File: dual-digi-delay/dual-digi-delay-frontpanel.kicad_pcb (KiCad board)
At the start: 2 copper layers, 50.5 x 175 mm, 1 part

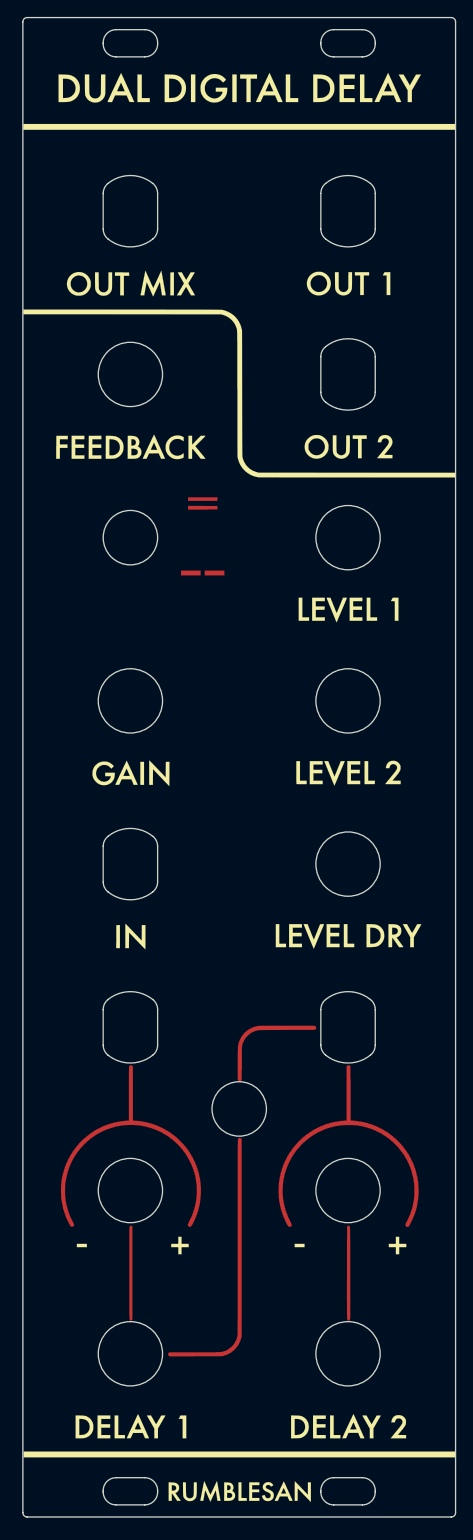
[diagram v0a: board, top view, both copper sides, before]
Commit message: Finalising rev 01 of dual digi delay
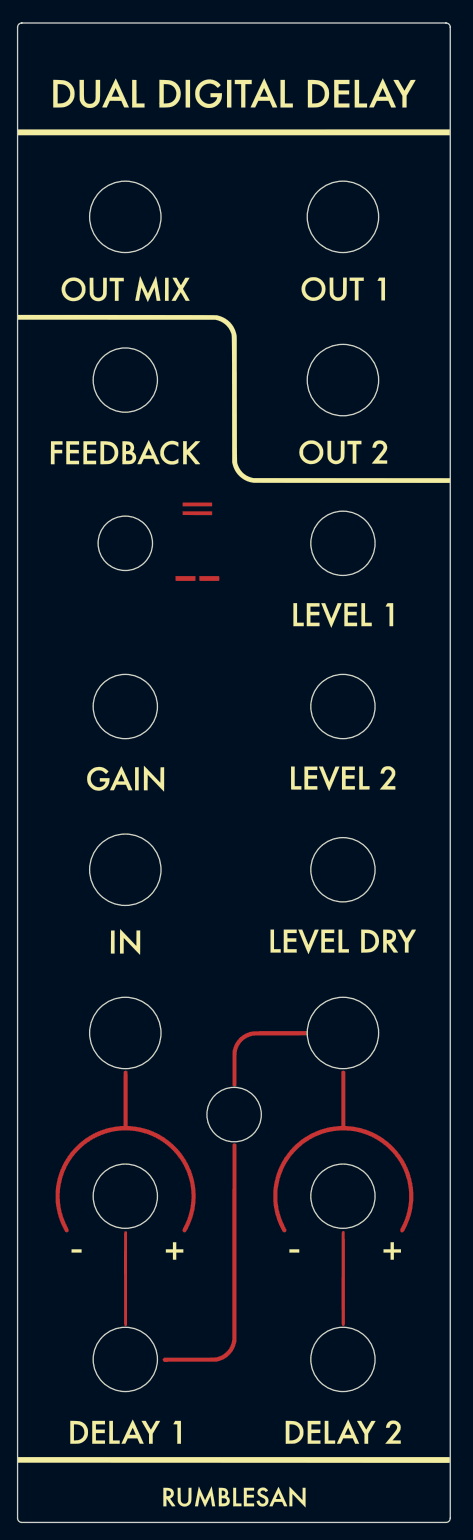
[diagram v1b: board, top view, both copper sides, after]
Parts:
- moved Ref** 0.89 mm to (102.2, 103.2)
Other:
- outline, holes or cut-outs redrawn
